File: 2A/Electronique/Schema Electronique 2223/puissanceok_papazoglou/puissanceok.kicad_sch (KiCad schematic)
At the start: 33 parts, among them J106 Conn_Phidget_PS_Stepper_1, J107 Conn_Phidget_PS_Stepper_2, J108 Conn_Phidget_PS_Stepper_3, J109 Conn_Phidget_PS_Stepper_4, J110 Conn_01x02, J111 Conn_GND, J112 Conn_GPIO_unused, J113 Conn_3.3V, J114 Conn_01x05, J115 Conn_01x05

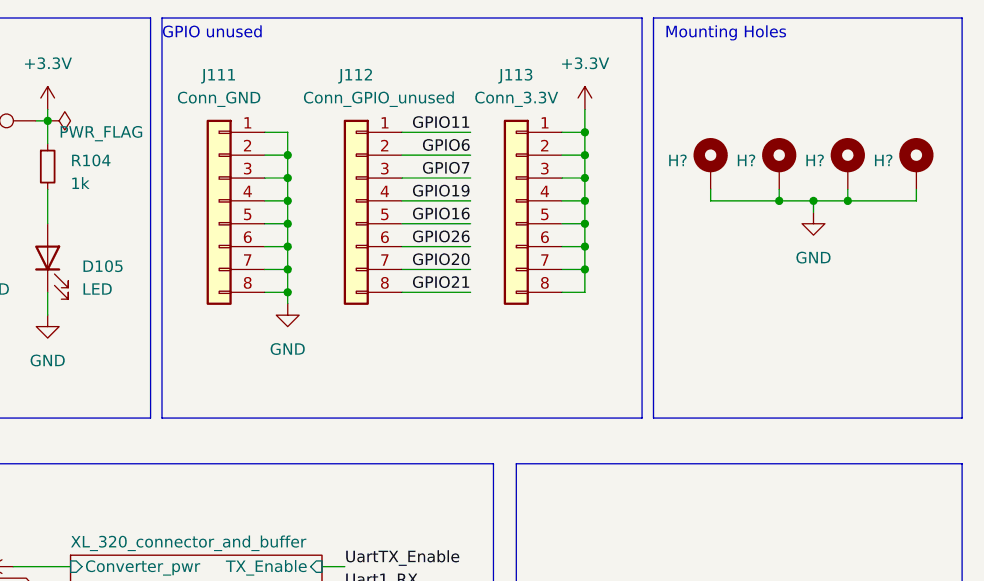
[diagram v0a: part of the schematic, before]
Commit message: update pcb
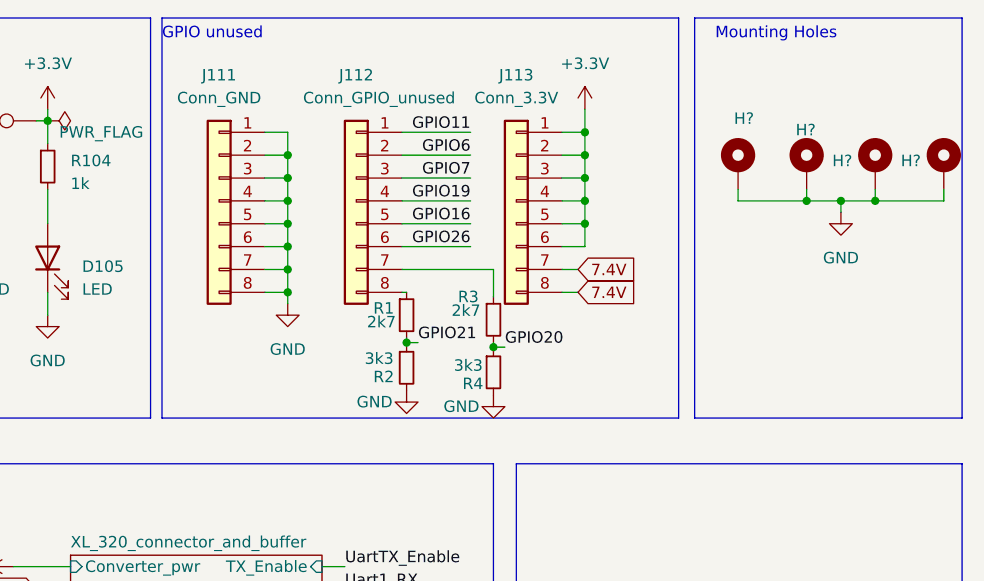
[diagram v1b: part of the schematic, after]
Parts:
- added R1, R3: 2k7, Resistor_SMD:R_0402_1005Metric, symbol Device:R_Small
- added R2, R4: 3k3, Resistor_SMD:R_0402_1005Metric, symbol Device:R_Small
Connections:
- net +3.3V: no longer J113.7 (Pin_7), J113.8 (Pin_8)
- net 7.4V: now also J113.7 (Pin_7), J113.8 (Pin_8)
- net GND: now also R2.2, R4.2
- net GPIO20: now also R3.2, R4.1; no longer J112.7 (Pin_7)
- net GPIO21: now also R1.2, R2.1; no longer J112.8 (Pin_8)
- new net: J112.7 (Pin_7), R3.1
- new net: J112.8 (Pin_8), R1.1
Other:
- moved on the sheet: H?
